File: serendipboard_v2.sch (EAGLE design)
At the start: 59 parts, among them IC1 TP4056, IC2 DW01A, IC3 DS3231/SO, Q1 FS8205A, Q2 DMP3056LSD, Q3 20V/0.2A/8MHz/1.2Ω/1Vth, Q4 20V/0.2A/8MHz/1.2Ω/1Vth, Q5 600mA/40V, Q6 TRANS_NPN-MMBT2222AL, U1 MAX17043, U2 AP2112-3.3, U3 AP2112-3.3, U4 9DoF IMU, U5 ESP32-WROOM-32D

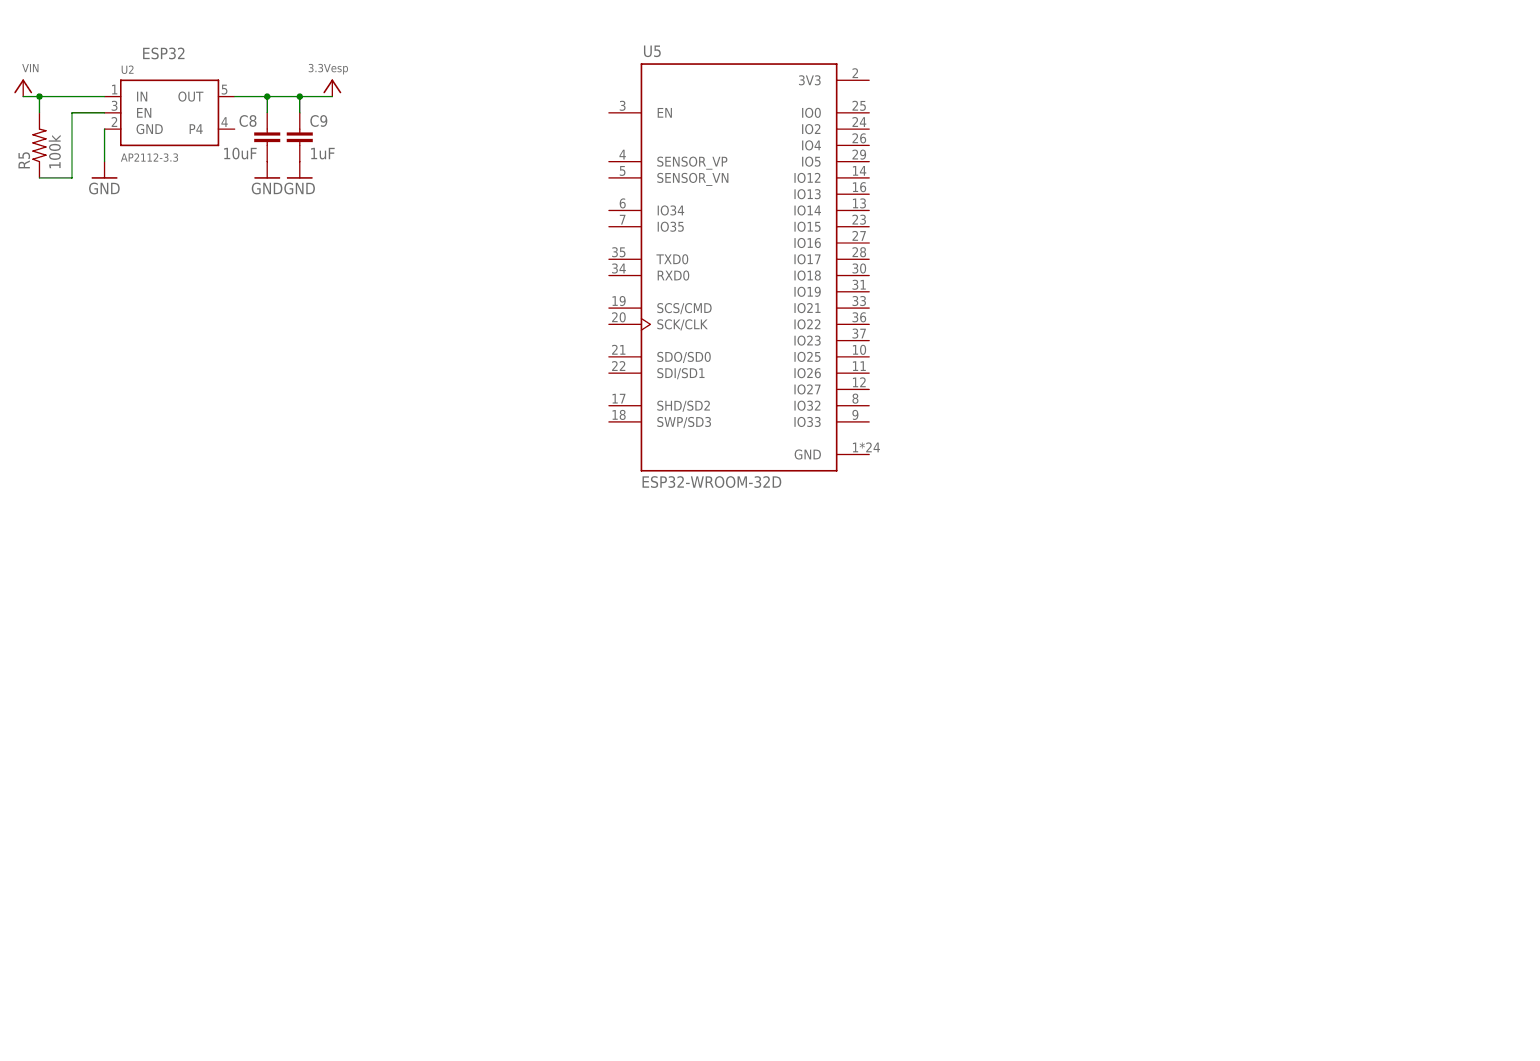
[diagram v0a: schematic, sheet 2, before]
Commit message: Update serendipboard_v2.sch
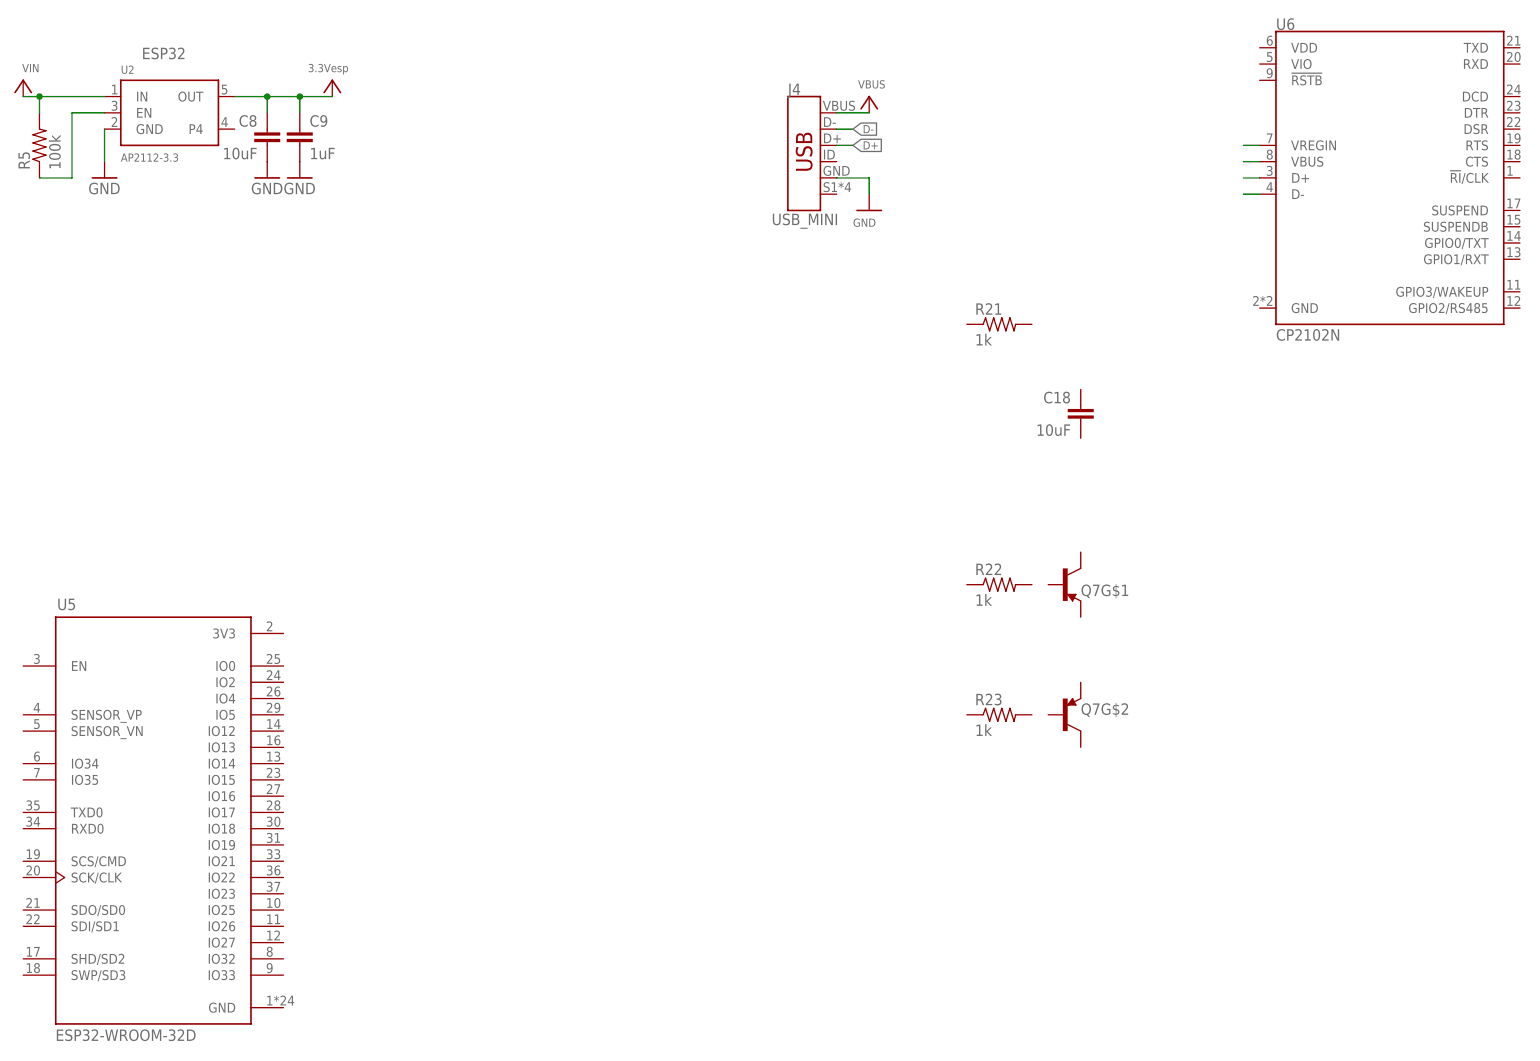
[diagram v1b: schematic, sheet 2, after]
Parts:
- added C18: 10uF, rcl:C-EUC0805
- added J4: USB_MINI, SparkFun-Connectors:USB_MINI-B_SMT
- added Q7: (no value), SparkFun-DiscreteSemi:TRANS_PNP_DUALSOT-363
- added R21, R22, R23: 1k, rcl:R-US_R0805
- added U6: CP2102N, SparkFun-IC-Comms:CP2102N
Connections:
- new net D+: J4.D+
- new net D-: J4.D-
- new net N$15: U6.D-
- new net N$16: U6.D+
- new net N$18: U6.VBUS
- new net N$19: U6.VREGIN
- net GND: now also J4.GND
- net VCC: now also J4.VBUS
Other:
- moved on the sheet: U5
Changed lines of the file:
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@@
 <part name="P+9" library="supply1" library_urn="urn:adsk.eagle:library:371" deviceset="VCC" device="" value="VIN"/>
 <part name="U5" library="ESP32-WROOM-32D" library_urn="urn:adsk.eagle:library:27379448" deviceset="ESP32-WROOM-32D" device="" package3d_urn="urn:adsk.eagle:package:27379451/1"/>
+<part name="U6" library="SparkFun-IC-Comms" deviceset="CP2102N" device=""/>
+<part name="J4" library="SparkFun-Connectors" deviceset="USB_MINI-B" device="_SMT" value="USB_MINI"/>
+<part name="R21" library="rcl" library_urn="urn:adsk.eagle:library:334" deviceset="R-US_" device="R0805" package3d_urn="urn:adsk.eagle:package:23553/2" value="1k"/>
+<part name="C18" library="rcl" library_urn="urn:adsk.eagle:library:334" deviceset="C-EU" device="C0805" package3d_urn="urn:adsk.eagle:package:23617/2" value="10uF"/>
+<part name="GND36" library="supply1" library_urn="urn:adsk.eagle:library:371" deviceset="GND" device=""/>
+<part name="P+29" library="supply1" library_urn="urn:adsk.eagle:library:371" deviceset="VCC" device="" value="VBUS"/>
+<part name="Q7" library="SparkFun-DiscreteSemi" deviceset="TRANS_PNP_DUAL" device="SOT-363" package3d_urn="urn:adsk.eagle:package:29757/2"/>
+<part name="R22" library="rcl" library_urn="urn:adsk.eagle:library:334" deviceset="R-US_" device="R0805" package3d_urn="urn:adsk.eagle:package:23553/2" value="1k"/>
+<part name="R23" library="rcl" library_urn="urn:adsk.eagle:library:334" deviceset="R-US_" device="R0805" package3d_urn="urn:adsk.eagle:package:23553/2" value="1k"/>
 </parts>
 <sheets>
@@
 <attribute name="VALUE" x="15.24" y="167.64" size="1.27" layer="96" rot="R180"/>
 </instance>
-<instance part="U5" gate="G$1" x="124.46" y="137.16" smashed="yes">
-<attribute name="NAME" x="109.4241" y="168.7545" size="1.778" layer="95"/>
-<attribute name="VALUE" x="109.1733" y="101.4919" size="1.778" layer="96"/>
+<instance part="U5" gate="G$1" x="33.02" y="50.8" smashed="yes">
+<attribute name="NAME" x="17.9841" y="82.3945" size="1.778" layer="95"/>
+<attribute name="VALUE" x="17.7333" y="15.1319" size="1.778" layer="96"/>
+</instance>
+<instance part="U6" gate="G$1" x="226.06" y="149.86" smashed="yes">
+<attribute name="NAME" x="208.28" y="172.974" size="1.778" layer="95"/>
+<attribute name="VALUE" x="208.28" y="124.46" size="1.778" layer="96"/>
+</instance>
+<instance part="J4" gate="G$1" x="134.62" y="152.4" smashed="yes">
+<attribute name="VALUE" x="129.54" y="142.494" size="1.778" layer="96" font="vector" rot="MR180" align="top-left"/>
+<attribute name="NAME" x="132.08" y="162.814" size="1.778" layer="95" font="vector"/>
+</instance>
+<instance part="R21" gate="G$1" x="165.1" y="127" smashed="yes">
+<attribute name="NAME" x="161.29" y="128.4986" size="1.778" layer="95"/>
+<attribute name="VALUE" x="161.29" y="123.698" size="1.778" layer="96"/>
+</instance>
+<instance part="C18" gate="G$1" x="177.8" y="114.3" smashed="yes" rot="MR0">
+<attribute name="NAME" x="176.276" y="114.681" size="1.778" layer="95" rot="MR0"/>
+<attribute name="VALUE" x="176.276" y="109.601" size="1.778" layer="96" rot="MR0"/>
+</instance>
+<instance part="GND36" gate="1" x="144.78" y="144.78" smashed="yes">
+<attribute name="VALUE" x="142.24" y="142.24" size="1.27" layer="96"/>
+</instance>
+<instance part="P+29" gate="VCC" x="144.78" y="162.56" smashed="yes">
+<attribute name="VALUE" x="147.32" y="165.1" size="1.27" layer="96" rot="R180"/>
+</instance>
+<instance part="Q7" gate="G$1" x="175.26" y="86.36" smashed="yes" rot="MR180">
+<attribute name="NAME" x="177.8" y="86.36" size="1.778" layer="95" font="vector" rot="MR180"/>
+<attribute name="VALUE" x="177.8" y="86.614" size="1.778" layer="96" font="vector" rot="MR180" align="top-left"/>
+</instance>
+<instance part="Q7" gate="G$2" x="175.26" y="66.04" smashed="yes">
+<attribute name="NAME" x="177.8" y="66.04" size="1.778" layer="95" font="vector"/>
+<attribute name="VALUE" x="177.8" y="65.786" size="1.778" layer="96" font="vector" align="top-left"/>
+</instance>
+<instance part="R22" gate="G$1" x="165.1" y="86.36" smashed="yes">
+<attribute name="NAME" x="161.29" y="87.8586" size="1.778" layer="95"/>
+<attribute name="VALUE" x="161.29" y="83.058" size="1.778" layer="96"/>
+</instance>
+<instance part="R23" gate="G$1" x="165.1" y="66.04" smashed="yes">
+<attribute name="NAME" x="161.29" y="67.5386" size="1.778" layer="95"/>
+<attribute name="VALUE" x="161.29" y="62.738" size="1.778" layer="96"/>
 </instance>
 </instances>
@@
 <pinref part="GND16" gate="1" pin="GND"/>
 <pinref part="C9" gate="G$1" pin="2"/>
+</segment>
+<segment>
+<pinref part="J4" gate="G$1" pin="GND"/>
+<wire x1="139.7" y1="149.86" x2="144.78" y2="149.86" width="0.1524" layer="91"/>
+<wire x1="144.78" y1="149.86" x2="144.78" y2="147.32" width="0.1524" layer="91"/>
+<pinref part="GND36" gate="1" pin="GND"/>
 </segment>
 </net>
@@
 <pinref part="P+9" gate="VCC" pin="VCC"/>
 </segment>
+<segment>
+<pinref part="J4" gate="G$1" pin="VBUS"/>
+<wire x1="139.7" y1="160.02" x2="144.78" y2="160.02" width="0.1524" layer="91"/>
+<pinref part="P+29" gate="VCC" pin="VCC"/>
+</segment>
 </net>
 <net name="N$8" class="0">
@@
 </segment>
 </net>
+<net name="D-" class="0">
+<segment>
+<pinref part="J4" gate="G$1" pin="D-"/>
+<wire x1="139.7" y1="157.48" x2="142.24" y2="157.48" width="0.1524" layer="91"/>
+<label x="142.24" y="157.48" size="1.27" layer="95" xref="yes"/>
+</segment>
+</net>
+<net name="D+" class="0">
+<segment>
+<pinref part="J4" gate="G$1" pin="D+"/>
+<wire x1="139.7" y1="154.94" x2="142.24" y2="154.94" width="0.1524" layer="91"/>
+<label x="142.24" y="154.94" size="1.27" layer="95" xref="yes"/>
+</segment>
+</net>
+<net name="N$15" class="0">
+<segment>
+<pinref part="U6" gate="G$1" pin="D-"/>
+<wire x1="205.74" y1="147.32" x2="203.2" y2="147.32" width="0.1524" layer="91"/>
+</segment>
+</net>
+<net name="N$16" class="0">
+<segment>
+<pinref part="U6" gate="G$1" pin="D+"/>
+<wire x1="205.74" y1="149.86" x2="203.2" y2="149.86" width="0.1524" layer="91"/>
+</segment>
+</net>
+<net name="N$18" class="0">
+<segment>
+<pinref part="U6" gate="G$1" pin="VBUS"/>
+<wire x1="205.74" y1="152.4" x2="203.2" y2="152.4" width="0.1524" layer="91"/>
+</segment>
+</net>
+<net name="N$19" class="0">
+<segment>
+<pinref part="U6" gate="G$1" pin="VREGIN"/>
+<wire x1="205.74" y1="154.94" x2="203.2" y2="154.94" width="0.1524" layer="91"/>
+</segment>
+</net>
